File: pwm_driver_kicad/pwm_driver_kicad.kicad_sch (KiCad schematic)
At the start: 11 parts, among them J1 Bornera, Q1 IRF1407, U1 NE555P

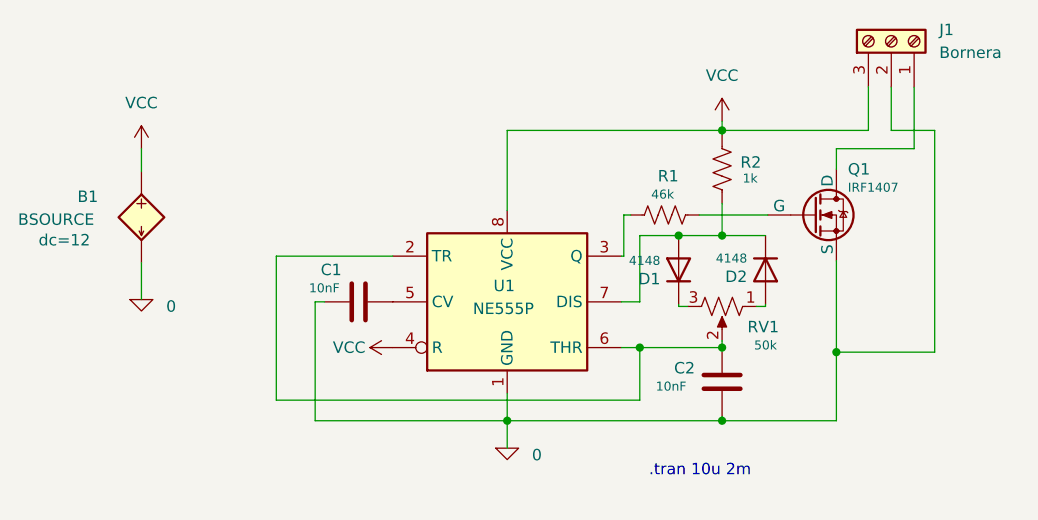
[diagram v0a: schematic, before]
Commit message: update schematic resistor values | fix simulation
NOTE: the pcb has **not** been updated yet
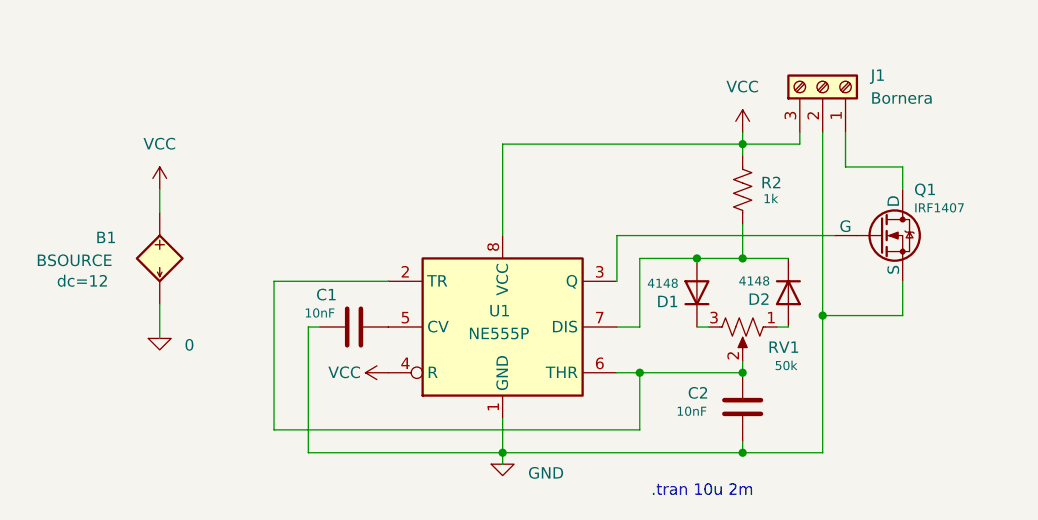
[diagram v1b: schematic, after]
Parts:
- removed R1: 46k, Resistor_THT:R_Axial_DIN0207_L6.3mm_D2.5mm_P7.62mm_Horizontal, symbol Device:R_US
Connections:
- net 0: no longer C1.2, C2.2, J1.2 (Pin_2), Q1.3 (S), U1.1 (GND)
- net at U1.3 (Q): now also Q1.2 (G)
- new net GND: C1.2, C2.2, J1.2 (Pin_2), Q1.3 (S), U1.1 (GND)
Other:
- moved on the sheet: B1, C1, C2, D1, D2, J1, Q1, R2, RV1, U1
